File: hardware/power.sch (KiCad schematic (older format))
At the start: 16 parts, among them J2 CONN_01X02, U11 SPX1117M3-L-3-3/TR, U2 ZXCT1107, U3 LM2576

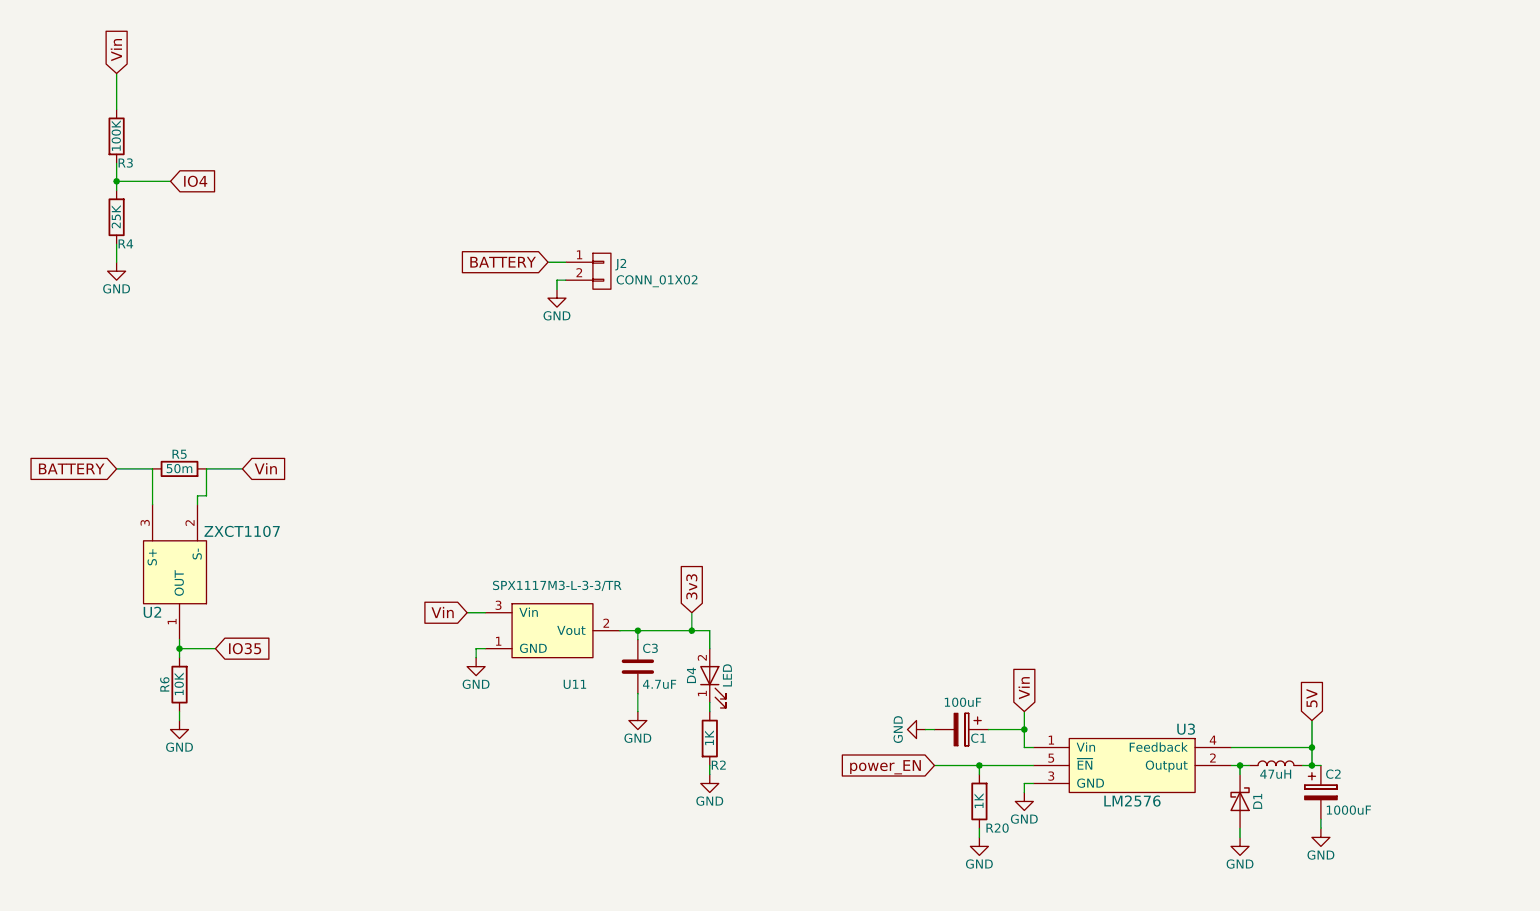
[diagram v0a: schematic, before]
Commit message: update
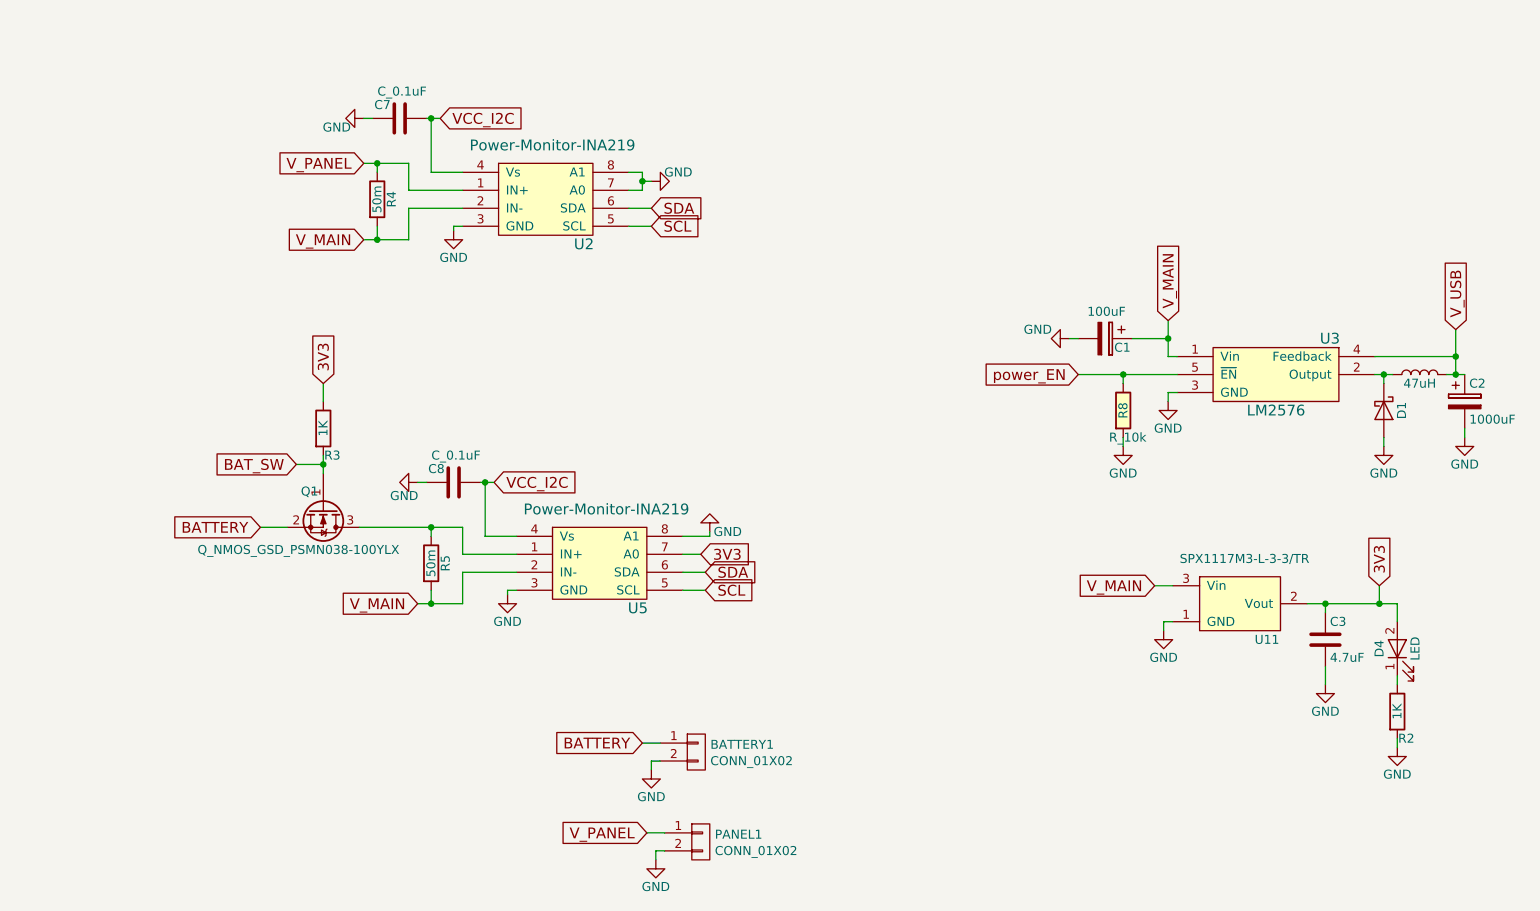
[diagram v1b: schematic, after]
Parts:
- removed R20: 1K, Resistors_SMD:R_0603_HandSoldering, symbol R
- removed R6: 10K, Resistors_SMD:R_0603_HandSoldering, symbol R
- removed U2: ZXCT1107, footprints:Current_sense-ZXCT1107, symbol ZXCT1107-RESCUE-5v-smart-solar-regulator
- added C7, C8: C_0.1uF, Capacitors_SMD:C_0603_HandSoldering, symbol C_0.1uF
- added PANEL1: CONN_01X02, open-automation:XT60, symbol CONN_01X02
- added Q1: Q_NMOS_GSD_PSMN038-100YLX, open-automation:SOT-669_PSMN038-100YLX, symbol Q_NMOS_GSD_PSMN038-100YLX
- added R8: R_10k, Resistors_SMD:R_0603_HandSoldering, symbol R_10k
- added U2, U5: Power-Monitor-INA219, TO_SOT_Packages_SMD:SOT-23-8_Handsoldering, symbol Power-Monitor-INA219
- BATTERY1: renamed from J2; footprint footprints:battery_input -> open-automation:XT60
- C1: footprint footprints:smd-cap-13.5 -> open-automation:CAP-RAD-5mm-UVR1H102MHD; Part Number EEV-FK1K101Q -> 860240675007
- C2: footprint footprints:smd-cap-13.5 -> open-automation:CAP-RAD-5mm-UVR1H102MHD; Part Number UUG1E102MNQ1MS -> UVR1H102MHD
- C3: footprint Capacitors_SMD:C_0603 -> Capacitors_SMD:C_0603_HandSoldering
- L1: footprint footprints:Inductor-SRR1210 -> open-automation:L-RAD-7.4mm; Part Number SRR1210-470M -> AIUR-06-470K
- R3: value 100K -> 1K; Part Number RC0603JR-07100KL -> RC0603JR-071KL
- R4: value 25K -> 50m; footprint Resistors_SMD:R_0603_HandSoldering -> Resistors_SMD:R_0805_HandSoldering; Part Number RC0603FR-0724K9L -> RL1220T-R050-J
- U11: footprint TO_SOT_Packages_SMD:SOT-223 -> open-automation:SPX1117M3; Part Number SPX1117M3-L-3-3/TR -> 1016-1848-1-ND
- U3: footprint footprints:Regulator-LM2576 -> open-automation:Regulator-LM2576
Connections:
- net BATTERY: now also Q1.2 (S); no longer R5.1
- net GND: now also C7.1, C8.1, PANEL1.2 (P2), R8.2, U2.3 (GND), U2.7 (A0), U2.8 (A1), U5.3 (GND), U5.8 (A1); no longer R4.1
- net power_EN: now also R8.1
- net 3v3 renamed 3V3
- net 3V3: now also R3.1, U5.7 (A0)
- net 5V renamed V_USB
- net IO4 renamed BAT_SW
- net BAT_SW: now also Q1.1 (G); no longer R4.2
- net Vin renamed V_MAIN
- net V_MAIN: now also R4.2, U2.2 (IN-), U5.2 (IN-); no longer R3.1
- new net: Q1.3 (D), R5.1, U5.1 (IN+)
- new net SCL: U2.5 (SCL), U5.5 (SCL)
- new net SDA: U2.6 (SDA), U5.6 (SDA)
- new net VCC_I2C: C7.2, C8.2, U2.4 (Vs), U5.4 (Vs)
- new net V_PANEL: PANEL1.1 (P1), R4.1, U2.1 (IN+)
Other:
- moved on the sheet: BATTERY1, C1, C2, C3, D1, D4, R2, R5, U11, U3
